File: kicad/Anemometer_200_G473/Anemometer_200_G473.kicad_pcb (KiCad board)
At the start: 2 copper layers, 23.3 x 37.9 mm, 86 parts, among them J1 Conn_01x01_Female, J10 Conn_01x01_Female, J11 USB_B_Micro, J12 Conn_01x01_Female, J13 Conn_01x01_Female, J14 Conn_01x01_Female, J15 Conn_01x01_Female, J16 Conn_01x01_Female, J17 Conn_01x01_Female, J18 Conn_01x01_Female, J19 Conn_01x01_Female, J2 Conn_01x01_Female, J20 Conn_01x01_Female, J21 Conn_01x01_Female, J3 Conn_01x08_Shielded, J4 Conn_01x01_Female, J5 Conn_01x01_Female, J6 Conn_01x01_Female, J7 Conn_01x01_Female, J8 Conn_01x04_Shielded, J9 Conn_01x01_Female, U1 W5500, U2 NCP1117-3.3, Y1 16, Y2 Crystal_GND24_Small

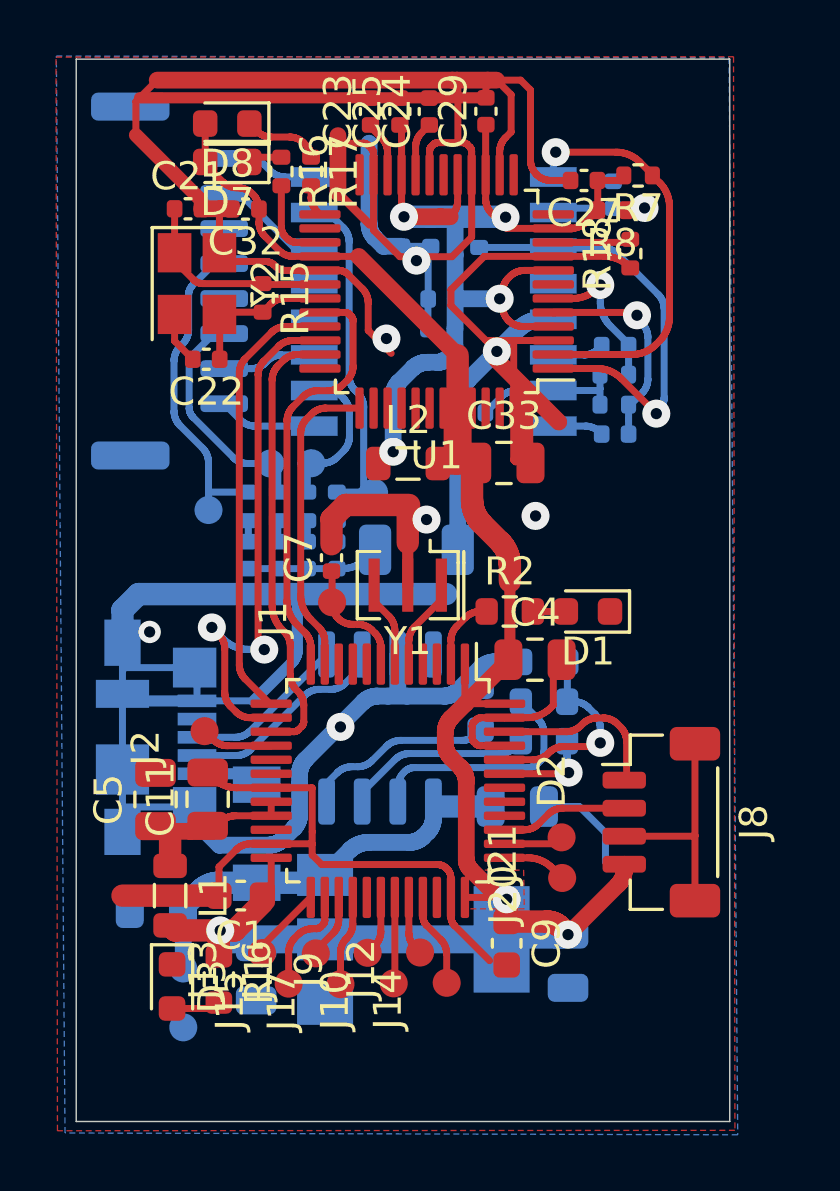
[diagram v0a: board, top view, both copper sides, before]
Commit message: изменено:      kicad/Anemometer_200_G473/Anemometer_200_G473-cache.lib 	изменено:      kicad/Anemometer_200_G473/Anemometer_200_G473.kicad_pcb 	изменено:      kicad/Anemometer_200_G473/Anemometer_200_G473.kicad_pcb-bak 	изменено:      kicad/Anemometer_200_G473/Anemometer_200_G473.sch 	изменено:      kicad/Anemometer_200_G473/Anemometer_200_G473.sch-bak
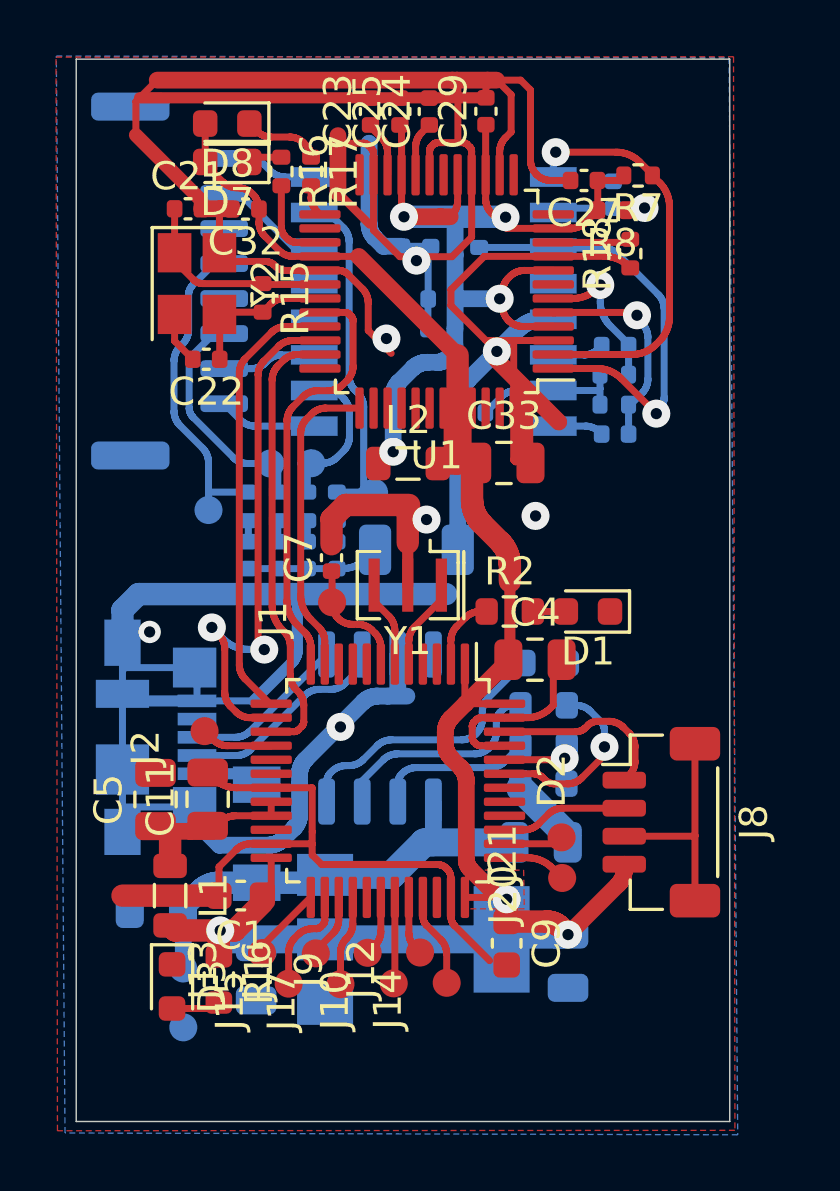
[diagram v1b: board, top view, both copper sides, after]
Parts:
- moved R5 4.34 mm to (33.9, 56.0)
- moved C8 2.80 mm to (33.9, 51.7), turned to 0 degrees
- moved R4 1.57 mm to (33.9, 54.7)
- moved C12 1.54 mm to (33.8, 58.1)
- moved R3 1.28 mm to (33.9, 53.2)
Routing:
- net GND: track 215.5 -> 209.7 mm
- net Net-(D2-Pad44): track 7.37 -> 3.64 mm
- net Net-(C8-Pad1): track 6.82 -> 9.87 mm
- net Net-(D5-Pad6): track 8.55 -> 5.62 mm
- net Net-(D2-Pad43): track 3.98 -> 6.72 mm
- net /+5v: track 15.2 -> 16.4 mm
- net Net-(D5-Pad7): track 6.68 -> 7.89 mm

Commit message: изменено:      kicad/Anemometer_200_G473/Anemometer_200_G473.kicad_pcb 	изменено:      kicad/Anemometer_200_G473/Anemometer_200_G473.kicad_sch
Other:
- net class Default removed
